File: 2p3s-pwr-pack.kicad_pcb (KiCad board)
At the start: 2 copper layers, 156.8 x 76.8 mm, 17 parts, among them P1 PAD, P10 PAD, P11 PAD, P12 PAD, P2 PAD, P3 PAD, P4 PAD, P5 PAD, P6 PAD, P7 PAD, P8 PAD, P9 PAD

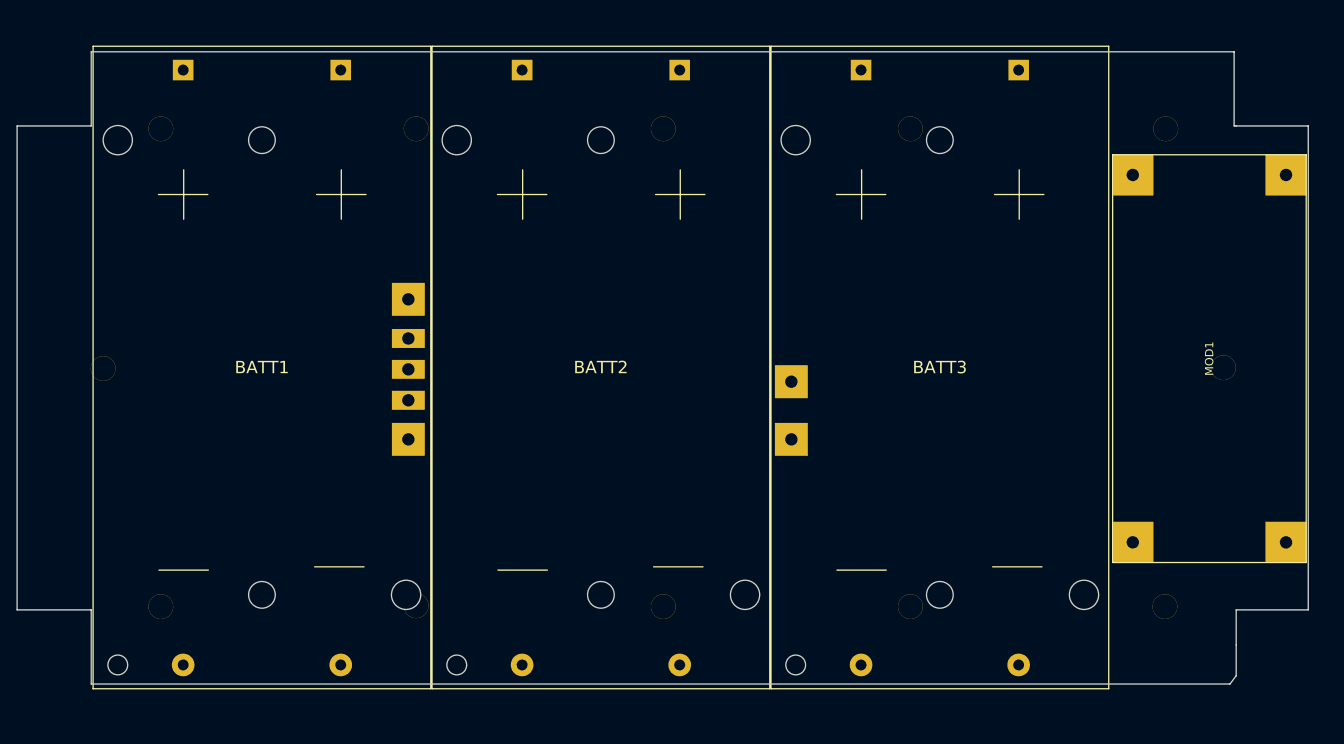
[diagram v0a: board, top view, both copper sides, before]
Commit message: 2019-03018 ready for ordering.
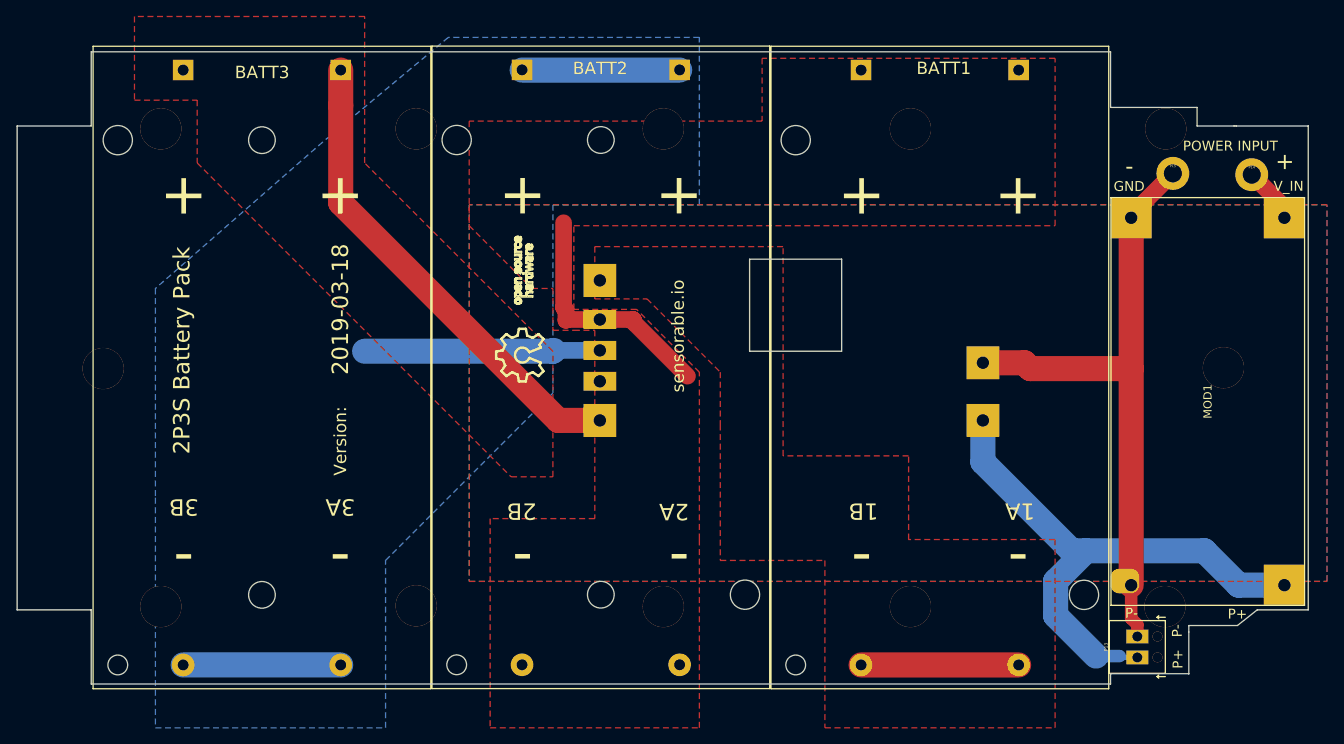
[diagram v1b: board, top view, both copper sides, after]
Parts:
- removed REF**: Module_BMS_Balancing_3s_AliExpress_BMS-3S0404LI502, Modulez:Module_BMS_Balancing_3s_AliExpress_BMS-3S0404LI502
- added MOD2: Module_AliExpress_BMS_3s_Balancing-3S0404LI502, Modulez:Module_BMS_Balancing_3s_AliExpress_BMS-3S0404LI502, B.Cu at (143.2, 101.5)
- added P13: Conn_Basic_2_pin, Footprints:TERM_BLK_2_SIDE_2.54MM, F.Cu at (185.2, 137.5)
- added P14: PAD, Footprints:HOLE_4mmx2.2mm, F.Cu at (199.1, 80.2)
- added P15: PAD, Footprints:HOLE_4mmx2.2mm, F.Cu at (189.6, 80.0)
- P1, P10, P11, P12, P2, P3, P4, P5, P6, P7, P8, P9: footprint NPTH_3mm -> NPTH_5mm
- moved MOD1 5.20 mm to (193.8, 107.7)
- renumbered BATT3 to BATT1, BATT1 to BATT3
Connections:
- BATT1 pad 2: GND1 -> Net-(BATT1-Pad2)
- BATT3 pad 1: Net-(BATT1-Pad1) (its old number) -> B+
- MOD1 pad 1: Net-(MOD1-Pad1) -> V_IN
- MOD1 pad 2: Net-(MOD1-Pad2) -> GND1
- MOD1 pad 3: Net-(MOD1-Pad3) -> GND1
- MOD1 pad 4: Net-(MOD1-Pad4) -> P+
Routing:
- net GND1: track 0.00 -> 76.9 mm
- net P+: track 0.00 -> 69.3 mm
- net Net-(BATT2-Pad1): track 0.00 -> 66.9 mm
- net B+: track 0.00 -> 58.5 mm
- net Net-(BATT1-Pad1): track 0.00 -> 29.8 mm
- net Net-(BATT1-Pad2): track 0.00 -> 19.1 mm
- net V_IN: track 0.00 -> 6.88 mm
- added copper zone on F.Cu, net B+
- added copper zone on B.Cu, net GND1
- added copper zone on F.Cu, net GND1
- added copper zone on F.Cu, net Net-(BATT1-Pad1)
- added copper zone on F.Cu, net Net-(BATT1-Pad2)
- added copper zone on B.Cu, net Net-(BATT2-Pad1)
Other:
- outline, holes or cut-outs redrawn
- board text added: "+"
- board text added: "-"
- board text added: "1A"
- board text added: "1B"
- board text added: "2019-03-18"
- board text added: "2A"
- board text added: "2B"
- board text added: "2P3S Battery Pack"
- board text added: "3A"
- board text added: "3B"
- board text added: "B+"
- board text added: "B-"
- board text added: "B1"
- board text added: "B2"
- board text added: "GND"
- board text added: "P+"
- board text added: "P-"
- board text added: "POWER INPUT"
- board text added: "V_IN"
- board text added: "Version:"
- board text added: "sensorable.io"
